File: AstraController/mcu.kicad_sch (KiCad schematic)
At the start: 8 parts, among them SW7 RESET, U5 ESP32-WROOM-32UE

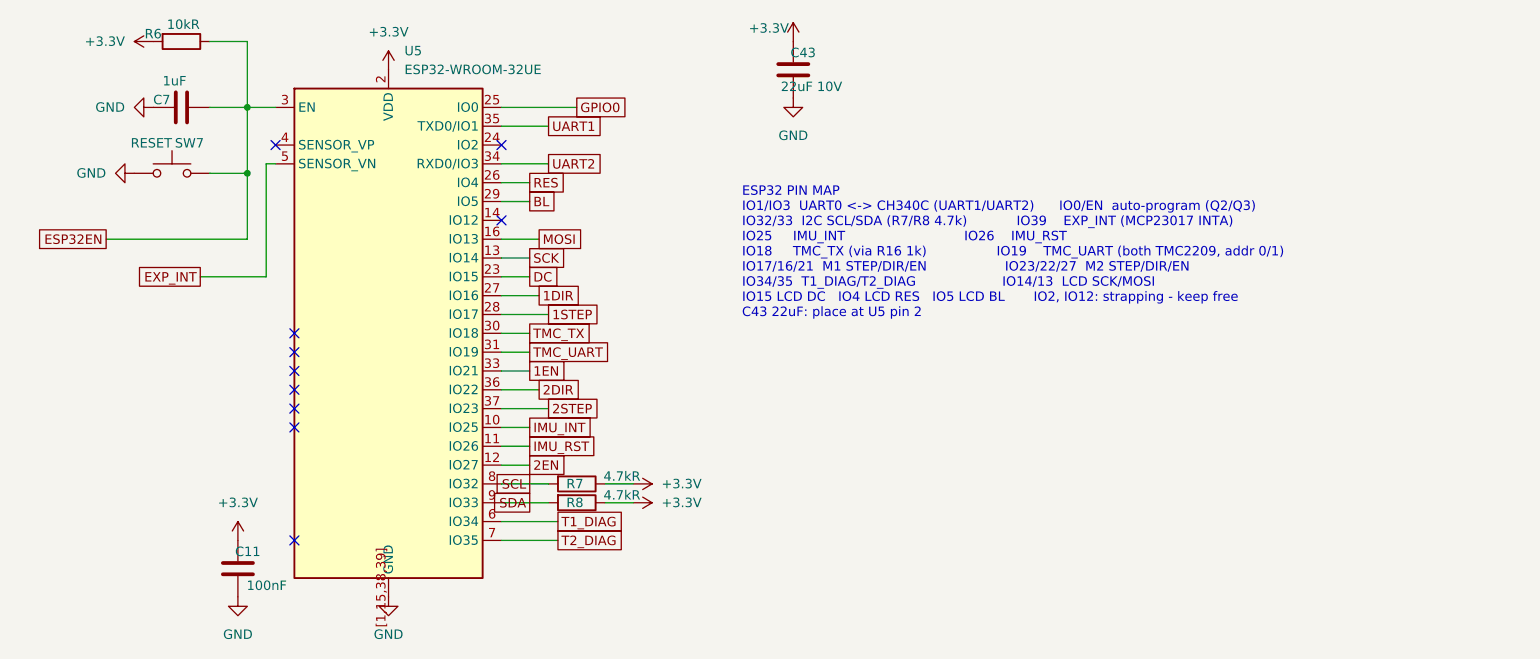
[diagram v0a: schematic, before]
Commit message: V0.7 pcb
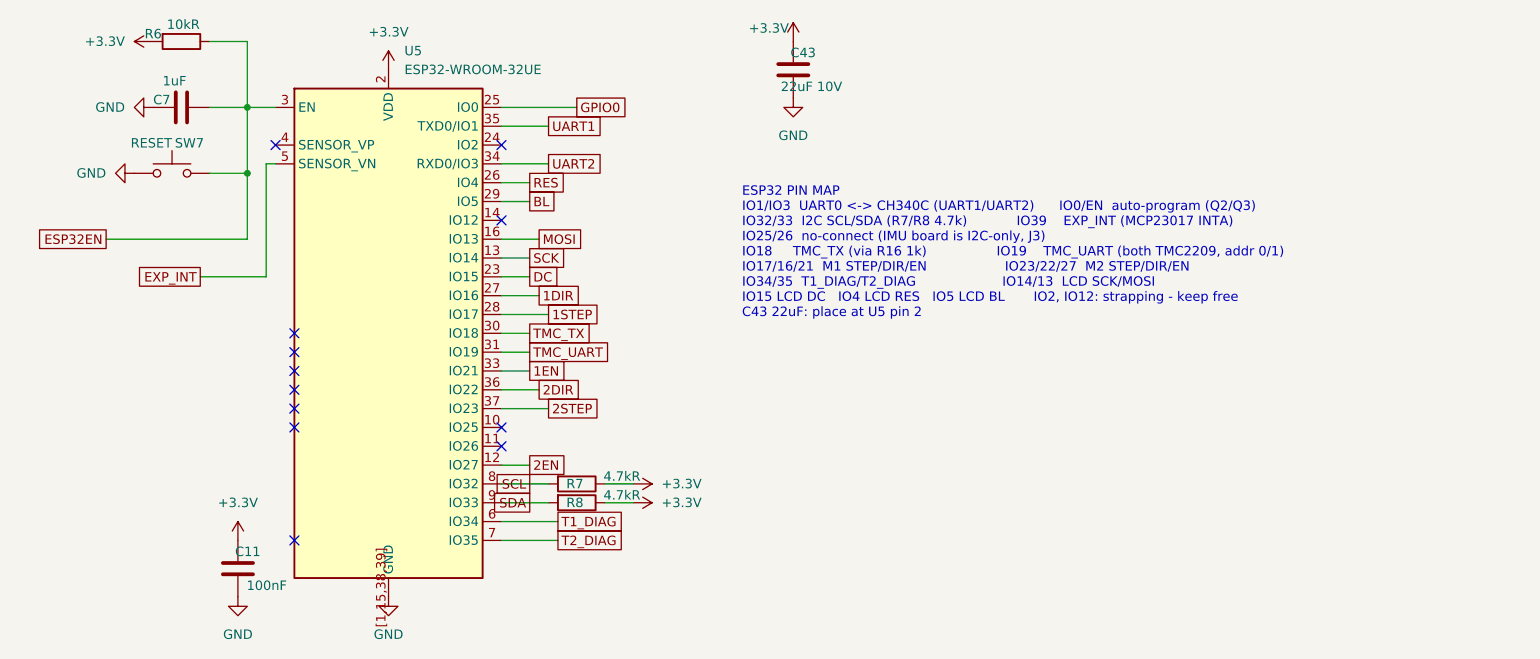
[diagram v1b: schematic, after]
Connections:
- net IMU_INT: no longer names the net of U5.10 (IO25)
- net IMU_RST: no longer names the net of U5.11 (IO26)
- no-connect marks 10 -> 12
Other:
- note added: "ESP32 PIN MAP IO1/IO3 UART0 <-> CH340C (UART1/UART2) IO0/EN auto-program (Q2/Q3) IO32/33 I2C SCL/SDA (R7/R8 4.7k) IO39 EXP_INT (MCP23017 INTA) IO25/26 no-connect (IMU board is I2C-only, J3) IO18 TMC_TX (via R16 1k) IO19 TMC_UART (both TMC2209, addr 0/1) IO17/16/21 M1 STEP/DIR/EN IO23/22/27 M2 STEP/DIR/EN IO34/35 T1_DIAG/T2_DIAG IO14/13 LCD SCK/MOSI IO15 LCD DC IO4 LCD RES IO5 LCD BL IO2, IO12: st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"
- note removed: "ESP32 PIN MAP IO1/IO3 UART0 <-> CH340C (UART1/UART2) IO0/EN auto-program (Q2/Q3) IO32/33 I2C SCL/SDA (R7/R8 4.7k) IO39 EXP_INT (MCP23017 INTA) IO25 IMU_INT IO26 IMU_RST IO18 TMC_TX (via R16 1k) IO19 TMC_UART (both TMC2209, addr 0/1) IO17/16/21 M1 STEP/DIR/EN IO23/22/27 M2 STEP/DIR/EN IO34/35 T1_DIAG/T2_DIAG IO14/13 LCD SCK/MOSI IO15 LCD DC IO4 LCD RES IO5 LCD BL IO2, IO12: strapping - keep free C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"
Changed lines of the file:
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@@
 	(wire
 		(pts
-			(xy 82.55 77.47) (xy 86.36 77.47)
+			(xy 43.18 34.29) (xy 48.26 34.29)
 		)
 		(stroke
@@
 	(wire
 		(pts
-			(xy 43.18 34.29) (xy 48.26 34.29)
+			(xy 82.55 85.09) (xy 88.9 85.09)
 		)
 		(stroke
@@
 	(wire
 		(pts
-			(xy 82.55 80.01) (xy 86.36 80.01)
+			(xy 82.55 72.39) (xy 87.63 72.39)
 		)
 		(stroke
@@
 	(wire
 		(pts
-			(xy 82.55 85.09) (xy 88.9 85.09)
+			(xy 48.26 34.29) (xy 52.07 34.29)
 		)
 		(stroke
@@
 	(wire
 		(pts
-			(xy 82.55 72.39) (xy 87.63 72.39)
+			(xy 29.21 52.07) (xy 48.26 52.07)
 		)
 		(stroke
@@
 	(wire
 		(pts
-			(xy 48.26 34.29) (xy 52.07 34.29)
+			(xy 48.26 34.29) (xy 48.26 25.4)
 		)
 		(stroke
@@
 	(wire
 		(pts
-			(xy 29.21 52.07) (xy 48.26 52.07)
+			(xy 82.55 52.07) (xy 87.63 52.07)
 		)
 		(stroke
@@
 		)
 	)
-	(wire
-		(pts
-			(xy 48.26 34.29) (xy 48.26 25.4)
-		)
-		(stroke
-			(width 0)
-			(type default)
-		)
-	)
-	(wire
-		(pts
-			(xy 82.55 52.07) (xy 87.63 52.07)
-		)
-		(stroke
-			(width 0)
-			(type default)
-		)
-	)
 	(global_label "1DIR"
 		(shape passive)
@@
 		)
 	)
-	(global_label "IMU_RST"
+	(global_label "SCK"
 		(shape passive)
-		(at 86.36 80.01 0)
+		(at 86.36 54.61 0)
 		(fields_autoplaced yes)
 		(effects
@@
 		)
 		(property "Intersheetrefs" "${INTERSHEET_REFS}"
-			(at 86.36 80.01 0)
-			(effects
-				(font
-					(size 1.27 1.27)
-				)
-				(justify left)
-				(hide yes)
-			)
-		)
-	)
-	(global_label "SCK"
-		(shape passive)
-		(at 86.36 54.61 0)
-		(fields_autoplaced yes)
-		(effects
-			(font
-				(size 1.27 1.27)
-			)
-			(justify left)
-		)
-		(property "Intersheetrefs" "${INTERSHEET_REFS}"
 			(at 86.36 54.61 0)
-			(effects
-				(font
-					(size 1.27 1.27)
-				)
-				(justify left)
-				(hide yes)
-			)
-		)
-	)
-	(global_label "IMU_INT"
-		(shape passive)
-		(at 86.36 77.47 0)
-		(fields_autoplaced yes)
-		(effects
-			(font
-				(size 1.27 1.27)
-			)
-			(justify left)
-		)
-		(property "Intersheetrefs" "${INTERSHEET_REFS}"
-			(at 86.36 77.47 0)
 			(effects
 				(font
@@
 	)
 	(no_connect
+		(at 82.55 77.47)
+	)
+	(no_connect
+		(at 82.55 80.01)
+	)
+	(no_connect
 		(at 52.07 39.37)
 	)
@@
 		)
 	)
-	(text "ESP32 PIN MAP\nIO1/IO3  UART0 <-> CH340C (UART1/UART2)      IO0/EN  auto-program (Q2/Q3)\nIO32/33  I2C SCL/SDA (R7/R8 4.7k)            IO39    EXP_INT (MCP23017 INTA)\nIO25     IMU_INT                             IO26    IMU_RST\nIO18     TMC_TX (via R16 1k)                 IO19    TMC_UART (both TMC2209, addr 0/1)\nIO17/16/21  M1 STEP/DIR/EN                   IO23/22/27  M2 STEP/DIR/EN\nIO34/35  T1_DIAG/T2_DIAG                     IO14/13  LCD SCK/MOSI\nIO15 LCD DC   IO4 LCD RES   IO5 LCD BL       IO2, IO12: strapping - keep free\nC43 22uF: place at U5 pin 2"
+	(text "ESP32 PIN MAP\nIO1/IO3  UART0 <-> CH340C (UART1/UART2)      IO0/EN  auto-program (Q2/Q3)\nIO32/33  I2C SCL/SDA (R7/R8 4.7k)            IO39    EXP_INT (MCP23017 INTA)\nIO25/26  no-connect (IMU board is I2C-only, J3)\nIO18     TMC_TX (via R16 1k)                 IO19    TMC_UART (both TMC2209, addr 0/1)\nIO17/16/21  M1 STEP/DIR/EN                   IO23/22/27  M2 STEP/DIR/EN\nIO34/35  T1_DIAG/T2_DIAG                     IO14/13  LCD SCK/MOSI\nIO15 LCD DC   IO4 LCD RES   IO5 LCD BL       IO2, IO12: strapping - keep free\nC43 22uF: place at U5 pin 2"
 		(exclude_from_sim no)
 		(at 115 45 0)
